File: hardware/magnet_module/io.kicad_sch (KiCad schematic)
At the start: 17 parts, among them J10 Conn_Coaxial, J11 Conn_Coaxial, J12 Conn_Coaxial, J13 Conn_Coaxial, J14 Conn_Coaxial, J15 Conn_Coaxial, J16 Conn_01x04_Pin, J17 Conn_01x04_Pin, J18 Conn_01x03_Pin, J19 Conn_01x03_Pin, U10 TXB0104RUT

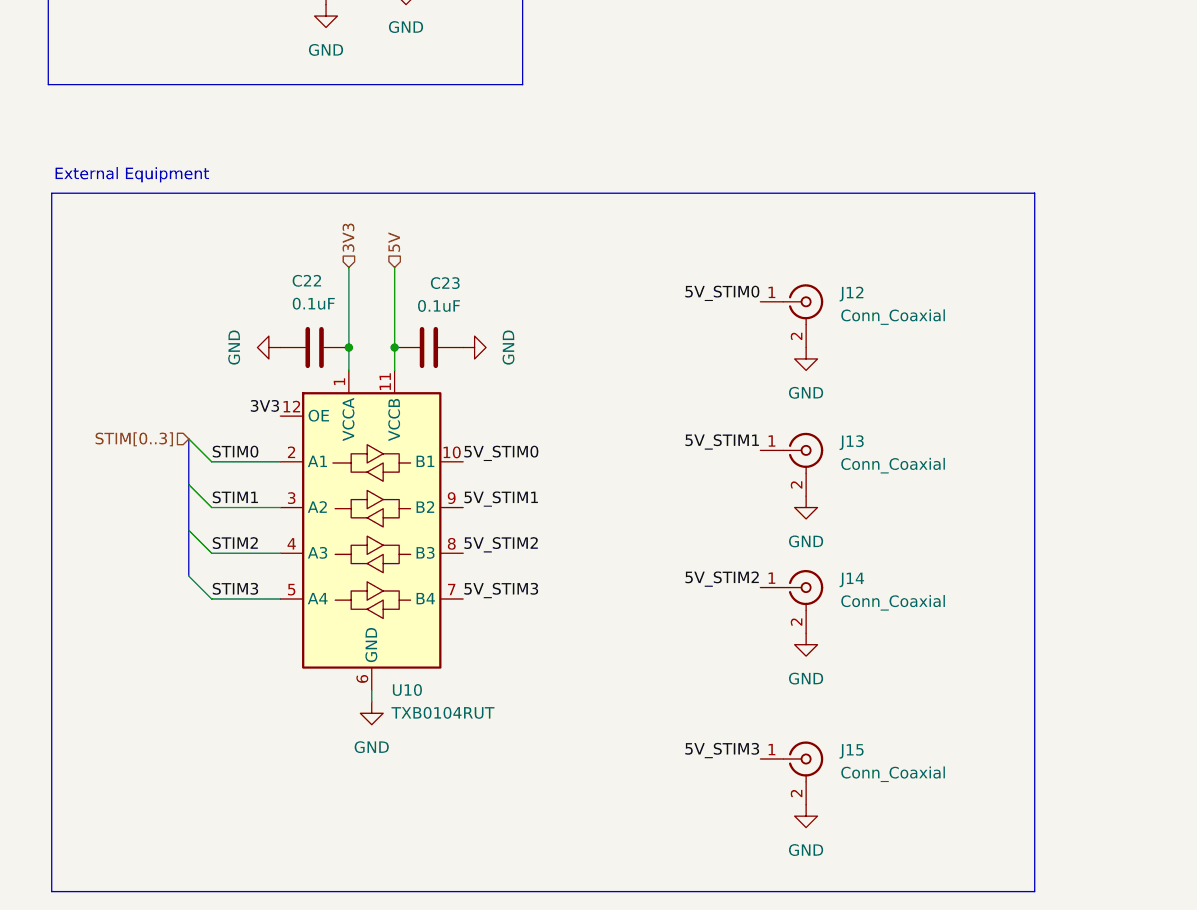
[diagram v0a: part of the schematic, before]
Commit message: make changes as requested by Ryan
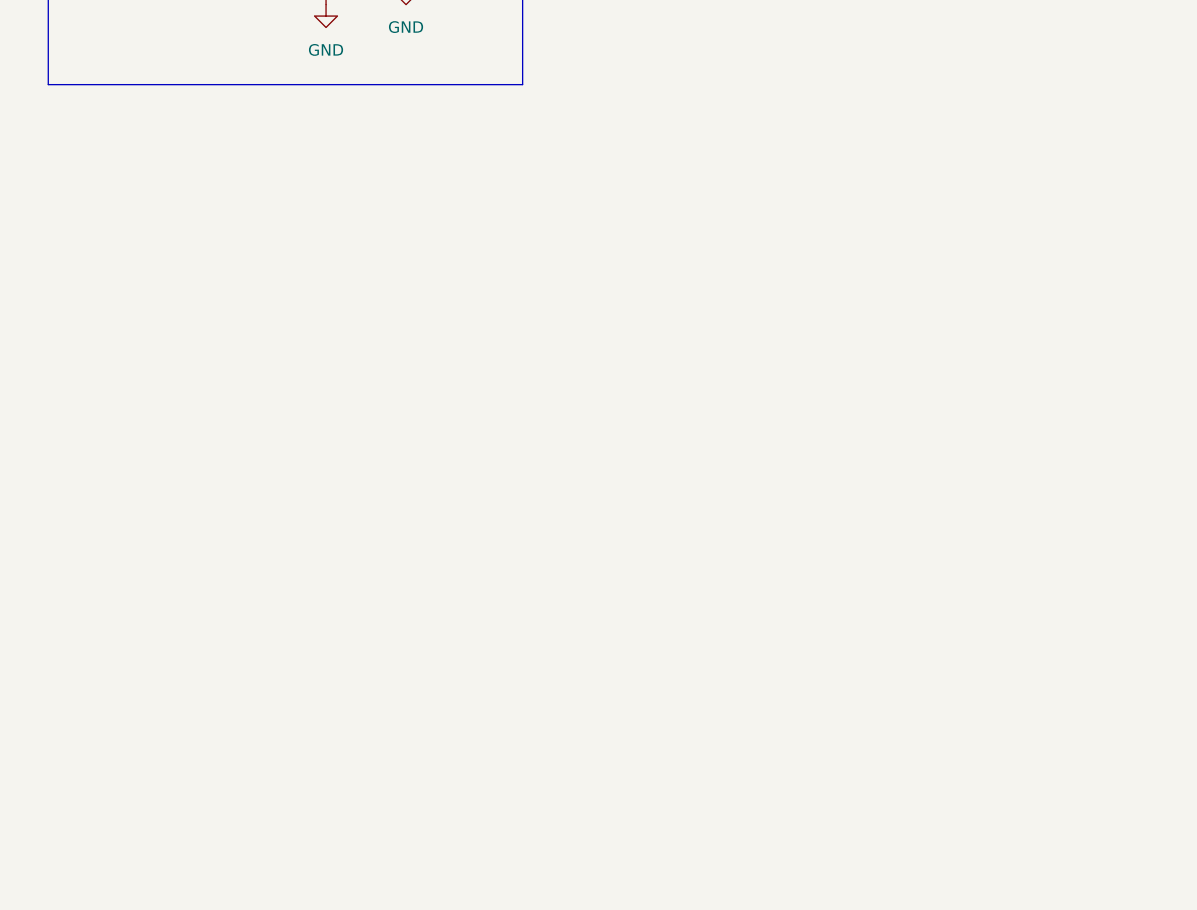
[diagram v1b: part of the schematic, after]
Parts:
- removed C22, C23: 0.1uF, Capacitor_SMD:C_0603_1608Metric, symbol Device:C
- removed J12, J13, J14, J15: Conn_Coaxial, symbol Connector:Conn_Coaxial
- removed U10: TXB0104RUT, Package_DFN_QFN:Texas_R-PUQFN-N12, symbol Logic_LevelTranslator:TXB0104RUT
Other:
- note removed: "External Equipment"
- company: Christie Lab, CU-Anschultz -> Christie Lab, CU-Anschutz
